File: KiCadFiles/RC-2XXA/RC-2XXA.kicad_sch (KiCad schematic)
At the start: 250 parts, among them J1 Conn_01x01_Pin, J2 Conn_01x04_Pin, J3 Conn_01x04_Pin, SW1 SW_DPST_x2, SW2 SW_DPST_x2, U1 TLV74318PDBVR, U2 PMW3360DM-T2QU, U3 TPD4E05U06DQAR, U4 STM32F072CBTx, U5 XC6206PxxxMR

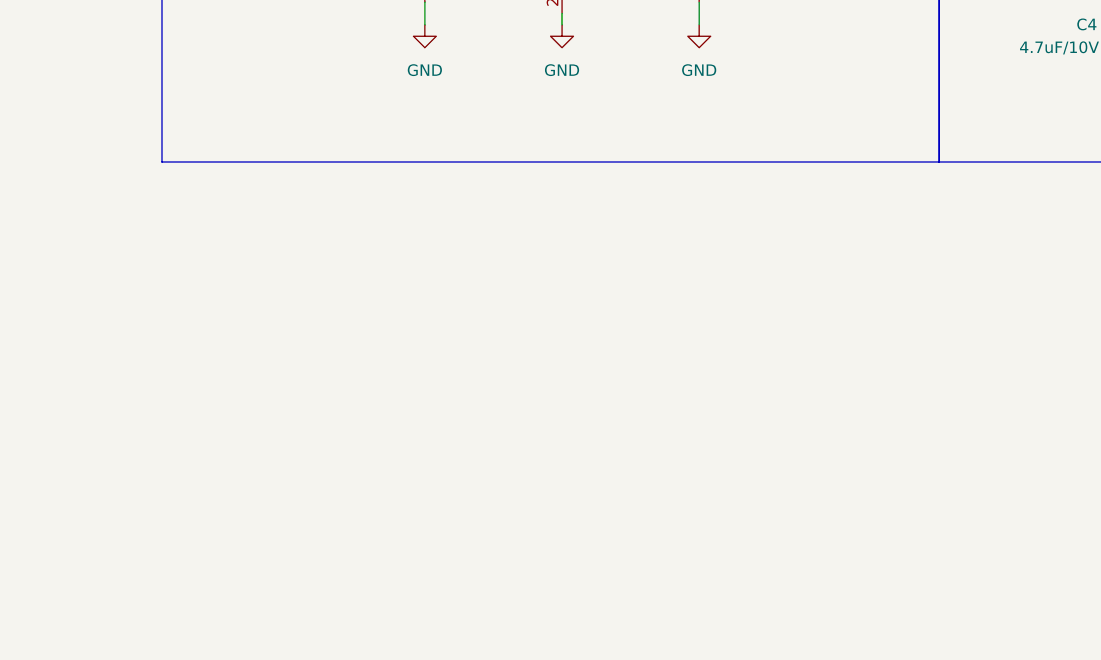
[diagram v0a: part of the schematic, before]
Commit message: Refactor code structure for improved readability and maintainability
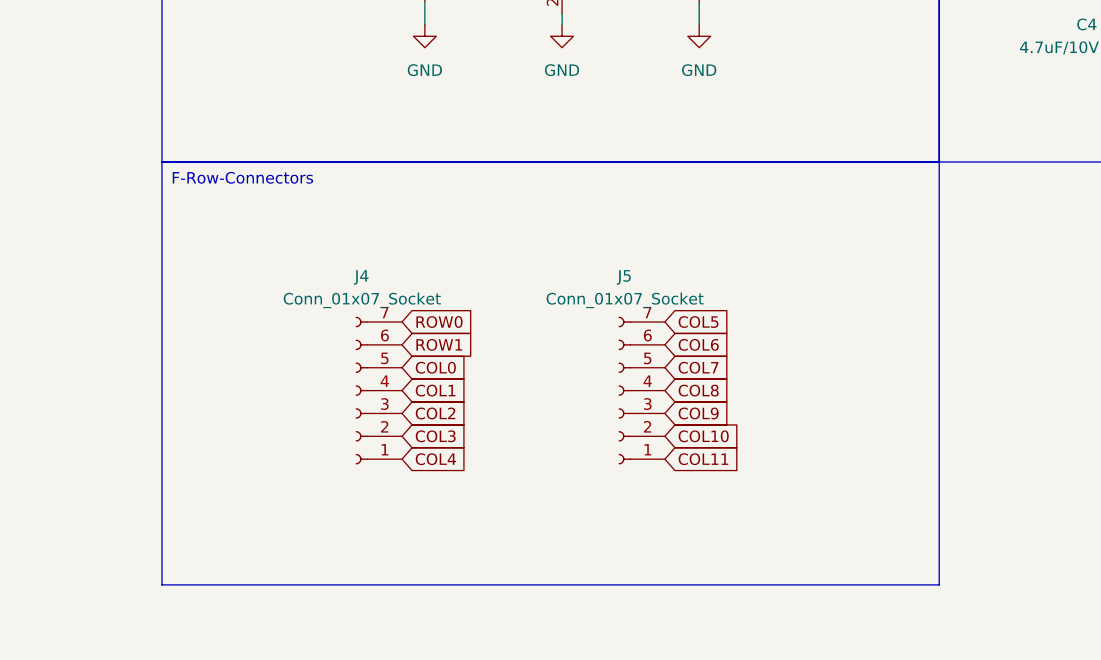
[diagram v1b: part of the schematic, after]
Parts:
- added J4, J5: Conn_01x07_Socket, Connector_JST:JST_SH_SM07B-SRSS-TB_1x07-1MP_P1.00mm_Horizontal, symbol Connector:Conn_01x07_Socket
- LED3: footprint My-Fi Footprints:DIP_LED_MX_3mm -> My-Fi Footprints:CAPS_LED_MX_3mm
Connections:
- net COL0: now also J4.5 (Pin_5)
- net COL1: now also J4.4 (Pin_4)
- net COL10: now also J5.2 (Pin_2)
- net COL11: now also J5.1 (Pin_1)
- net COL2: now also J4.3 (Pin_3)
- net COL3: now also J4.2 (Pin_2)
- net COL4: now also J4.1 (Pin_1)
- net COL5: now also J5.7 (Pin_7)
- net COL6: now also J5.6 (Pin_6)
- net COL7: now also J5.5 (Pin_5)
- net COL8: now also J5.4 (Pin_4)
- net COL9: now also J5.3 (Pin_3)
- net ROW0: now also J4.7 (Pin_7)
- net ROW1: now also J4.6 (Pin_6)
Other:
- note added: "F-Row-Connectors"
